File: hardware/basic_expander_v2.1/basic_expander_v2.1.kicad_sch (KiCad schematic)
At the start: 13 parts, among them J1 POD, SW1 SW_Push, SW2 SW_Push, SW3 SW_Push, SW4 SW_Push, SW5 SW_Push, SW6 SW_Push

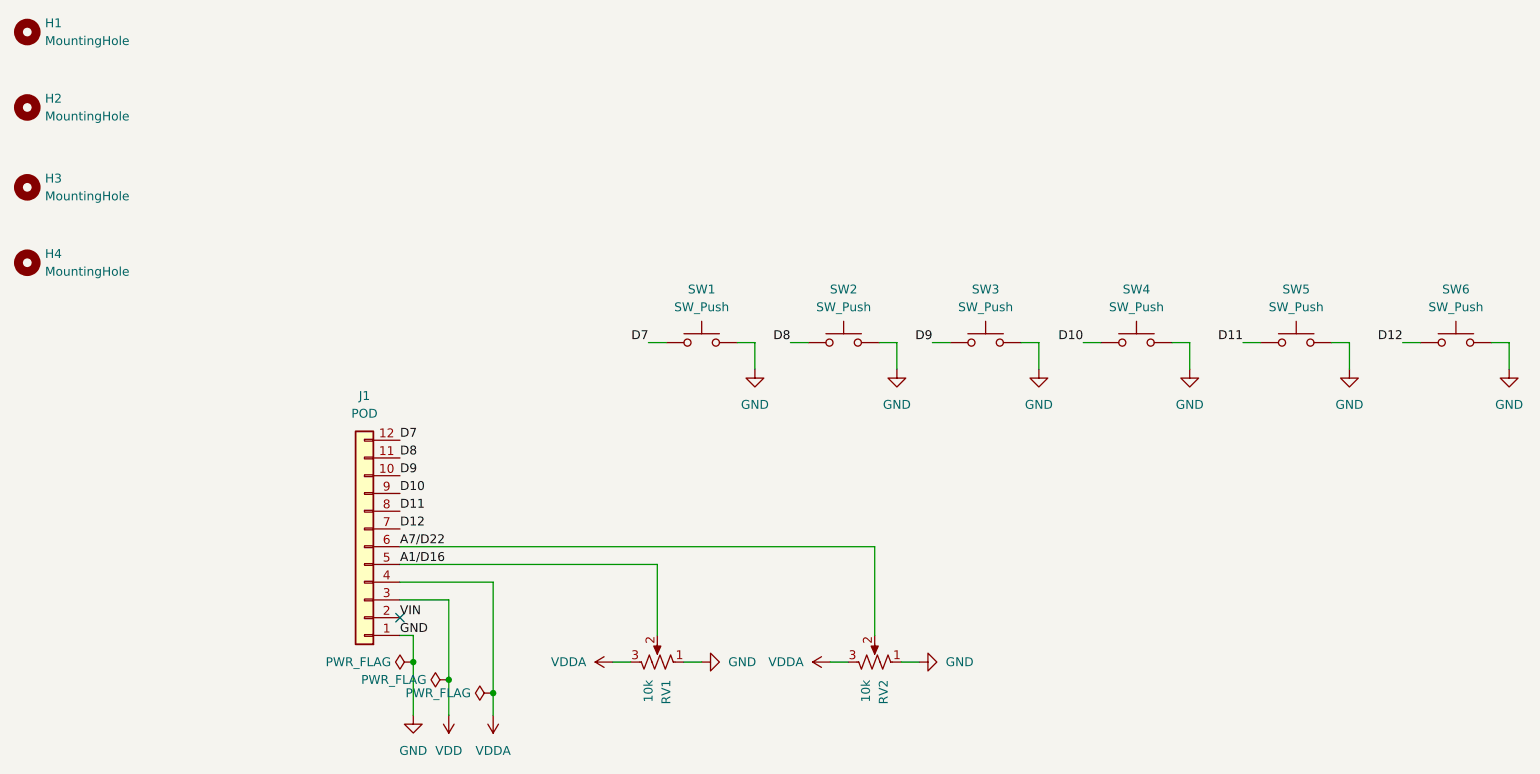
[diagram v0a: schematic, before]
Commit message: add v2.1 gerber files
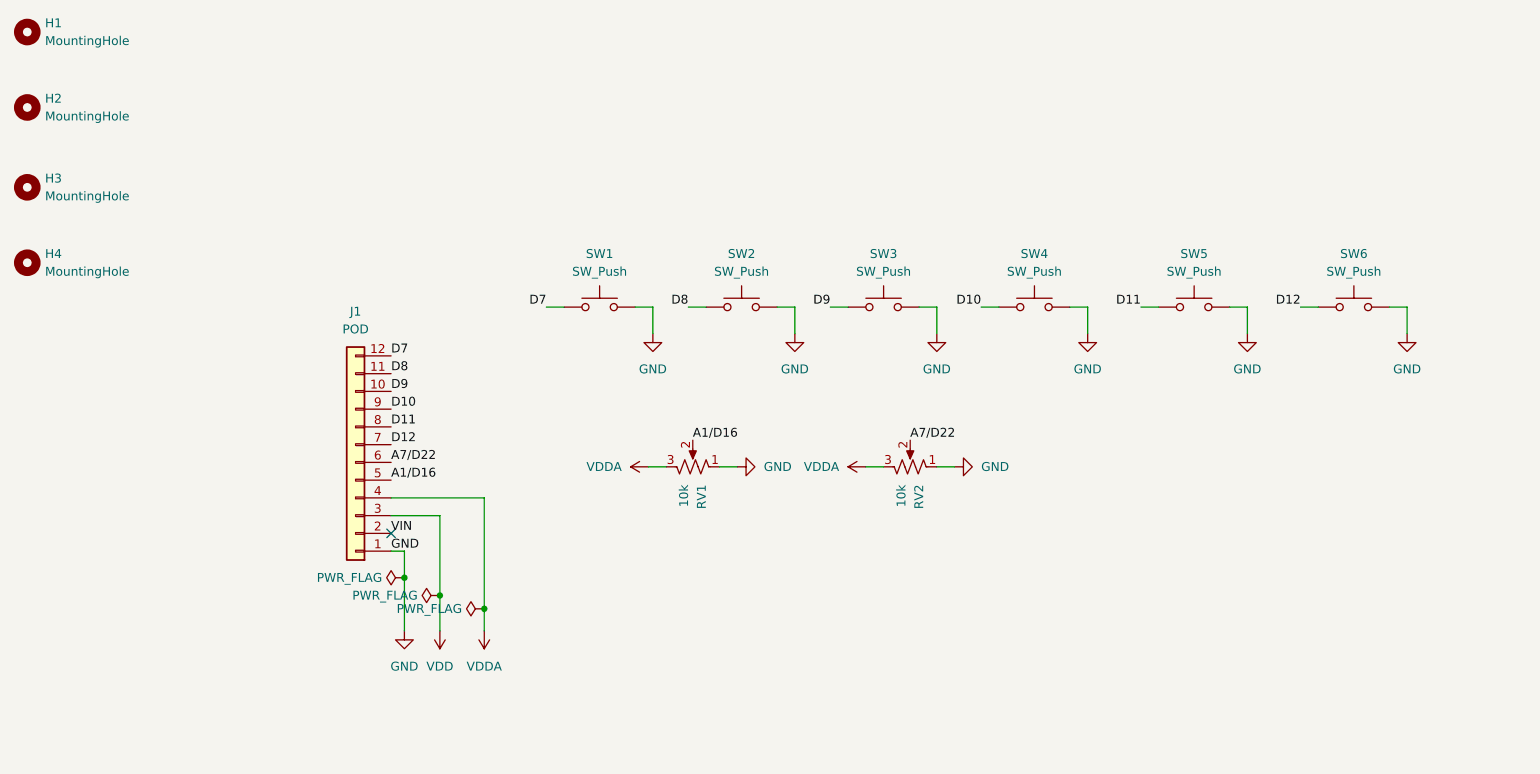
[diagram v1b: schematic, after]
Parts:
- RV1, RV2: footprint Potentiometer_THT:Potentiometer_Alpha_RD901F-40-00D_Single_Vertical -> Local:Potentiometer_uxcel_9mm_Single_Vertical
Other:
- moved on the sheet: J1, RV1, RV2, SW1, SW2, SW3, SW4, SW5, SW6
